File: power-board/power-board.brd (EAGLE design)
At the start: 77.1 x 43 mm, 25 parts

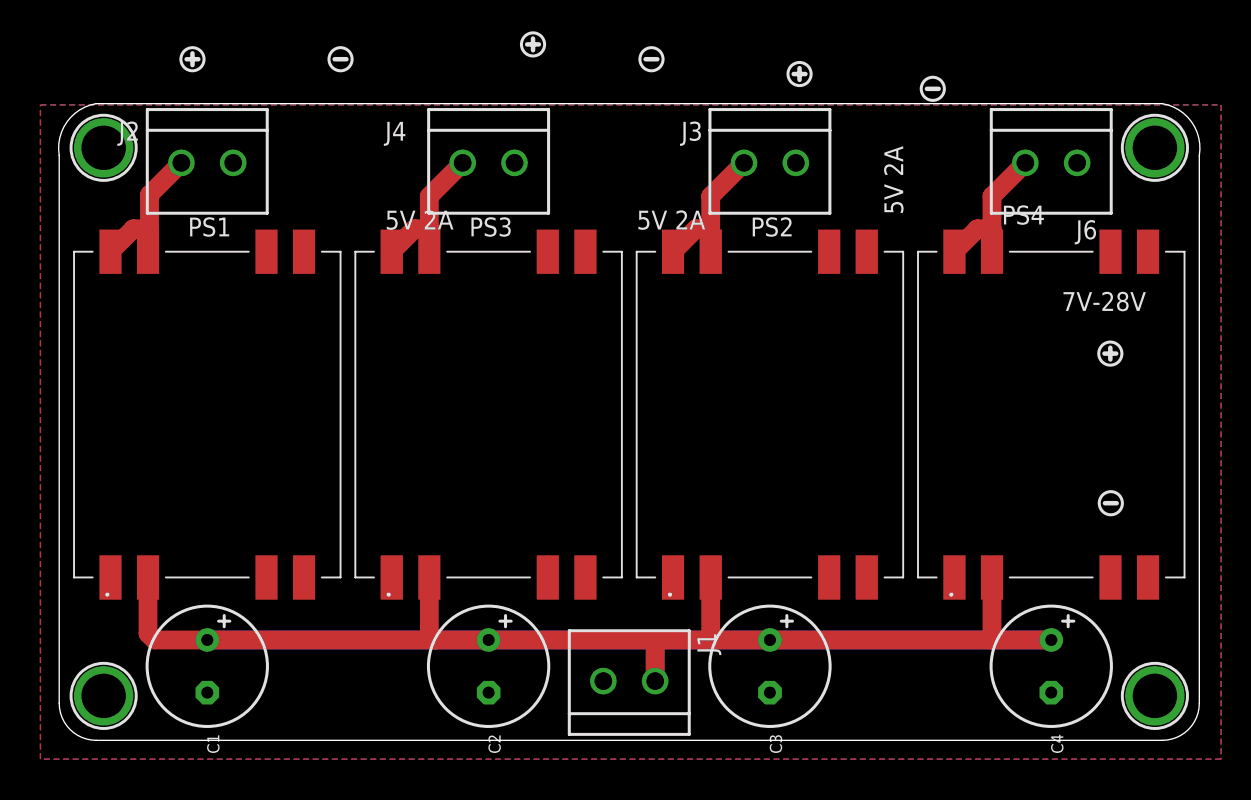
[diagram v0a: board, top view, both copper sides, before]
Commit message: Publish v1.0.0 Power Board and Power Bridge
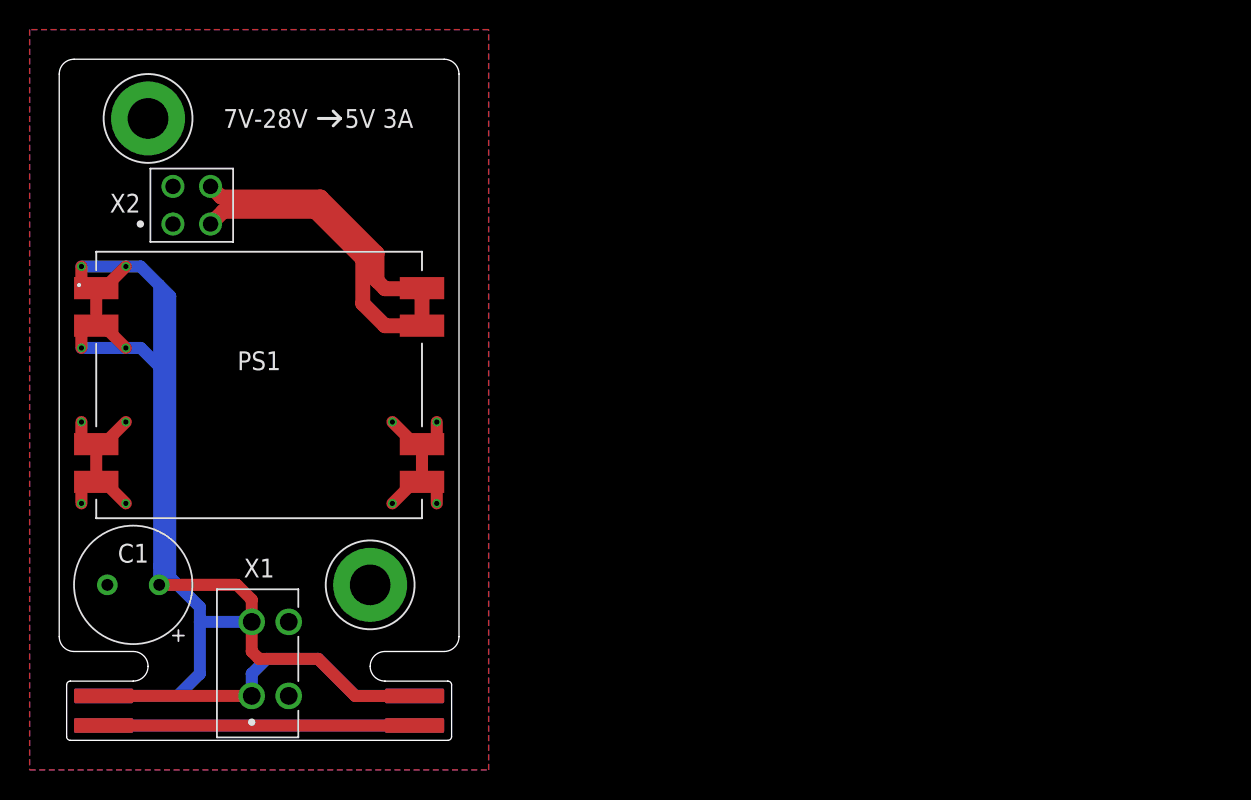
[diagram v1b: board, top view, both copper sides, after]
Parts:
- removed C2, C3, C4: (no value), sanisimov:CELEC_3.5MM_8MM
- removed J1, J2, J3, J4, J6: (no value), sanisimov:WR-TBL-1X2-3.5MM
- removed PS2, PS3, PS4: 5V, sanisimov:K8801
- removed U$1, U$4: MOUNTINGHOLE3.0THIN, sanisimov:MOUNTINGHOLE_3.0_PLATEDTHIN
- removed U$10, U$12, U$6, U$8: (no value), microbuilder:SYMBOL_MINUS
- removed U$11, U$5, U$7, U$9: (no value), microbuilder:SYMBOL_PLUS
- added X1: CON-FE02-1, _Library.b1f76137-4d0f-4ce2-9703-0cd83550450f.flbr:PTSM0,5/2-2,5-HTHRR24
- added X2: CON-FE02-2HDRVR4W64P254_2X2, _Library.b1f76137-4d0f-4ce2-9703-0cd83550450f.flbr:HDRVR4W64P254_2X2
- added X3, X4: CON-MA02-1, _Library.b1f76137-4d0f-4ce2-9703-0cd83550450f.flbr:AVX-BTB-009159002001106
- C1: value (none) -> CAP_ELECTROLYTIC; device sanisimov:CELEC_3.5MM_8MM -> _Library.b1f76137-4d0f-4ce2-9703-0cd83550450f.flbr:CAPPRD350W60D800H800B
- PS1: value 5V -> (none); device sanisimov:K8801 -> _Library.b1f76137-4d0f-4ce2-9703-0cd83550450f.flbr:K8801
- U$2, U$3: value MOUNTINGHOLE3.0THIN -> MOUNTINGHOLE2.7_THICK; device sanisimov:MOUNTINGHOLE_3.0_PLATEDTHIN -> _Library.b1f76137-4d0f-4ce2-9703-0cd83550450f.flbr:MOUNTINGHOLE_2.7_PLATED_THICK
- moved U$3 78.4 mm to (6.00, 42.0)
- moved U$2 19.5 mm to (21.0, 10.5)
- moved C1 7.43 mm to (5.00, 10.5), turned to 180 degrees
- moved PS1 4.03 mm to (13.5, 24.0), turned to 270 degrees
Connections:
- removed net N$3: J3.1, PS2.5, PS2.6
- removed net N$5: J4.1, PS3.5, PS3.6
- removed net N$7: J2.1, PS1.5, PS1.6
- removed net VCC: C1.+, C2.+, C3.+, C4.+, J1.1, PS1.1, PS1.2, PS2.1, PS2.2, PS3.1, PS3.2, PS4.1, PS4.2
- new net VIN: C1.1, PS1.1, PS1.2, X1.1, X1.2, X3.1, X3.3, X4.2, X4.4
- net GND: now also C1.2, X1.3, X1.4, X2.1, X2.2, X3.2, X3.4, X4.1, X4.3; no longer C1.-, C2.-, C3.-, C4.-, J1.2, J2.2, J3.2, J4.2, J6.2, PS2.3, PS2.4, PS2.7, PS2.8, PS3.3, PS3.4, PS3.7, PS3.8, PS4.3, PS4.4, PS4.7, PS4.8
- net N$1: now also PS1.5, PS1.6, X2.3, X2.4; no longer J6.1, PS4.5, PS4.6
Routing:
- net VCC: track 140.8 -> 0.00 mm
- net VIN: track 0.00 -> 132.5 mm, vias 0 -> 4
- net GND: track 0.00 -> 67.6 mm, vias 0 -> 8
- net N$1: track 10.1 -> 40.4 mm
- net N$7: track 10.2 -> 0.00 mm
- net N$3: track 10.1 -> 0.00 mm
- net N$5: track 10.1 -> 0.00 mm
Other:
- board size 77.1 x 43 mm -> 27 x 46 mm
- board text added: "7V-28V 5V 3A"
- board text removed: "5V 2A"
- board text removed: "7V-28V"
